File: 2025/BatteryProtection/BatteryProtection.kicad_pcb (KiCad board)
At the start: 2 copper layers, 58.4 x 140.1 mm, 57 parts, among them J1 Conn_01x02_Socket, J2 Conn_01x02_Pin, J3 Conn_01x02_Pin, Q1 IXTA140P05T, Q10 BC847, Q11 BC847, Q12 BC847, Q2 BC847, Q3 BC847, Q4 BC847, Q5 BC847, Q6 BC847, Q7 BC847, Q8 BC847, Q9 BC847, U1 MCP6561-OT, U2 MCP6561-OT, U3 MCP1799x-330xxTT

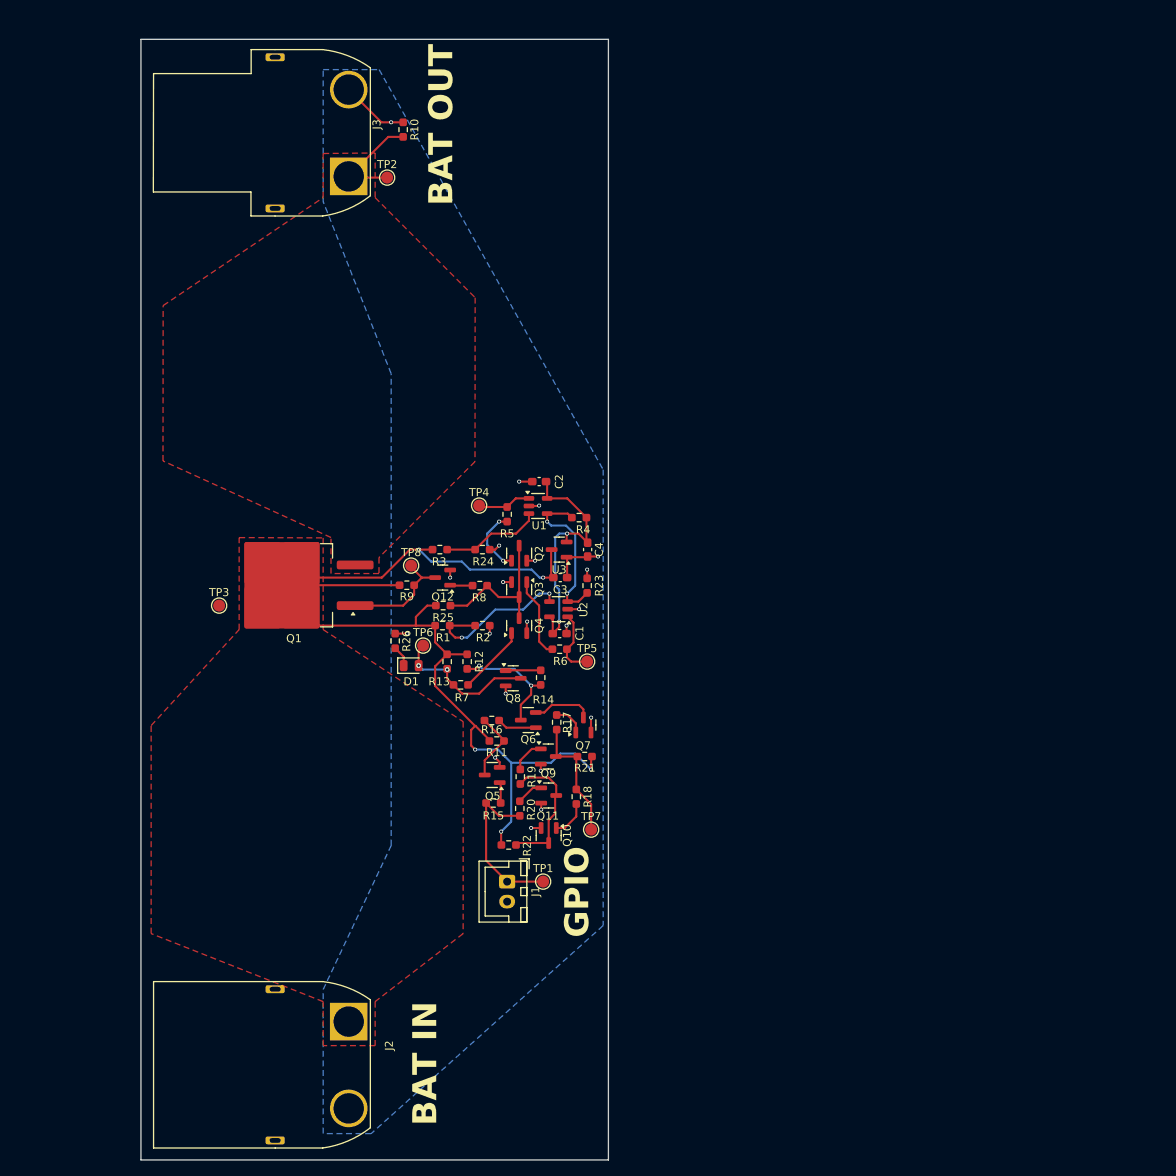
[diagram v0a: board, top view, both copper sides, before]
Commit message: DID the voltage protection PCB
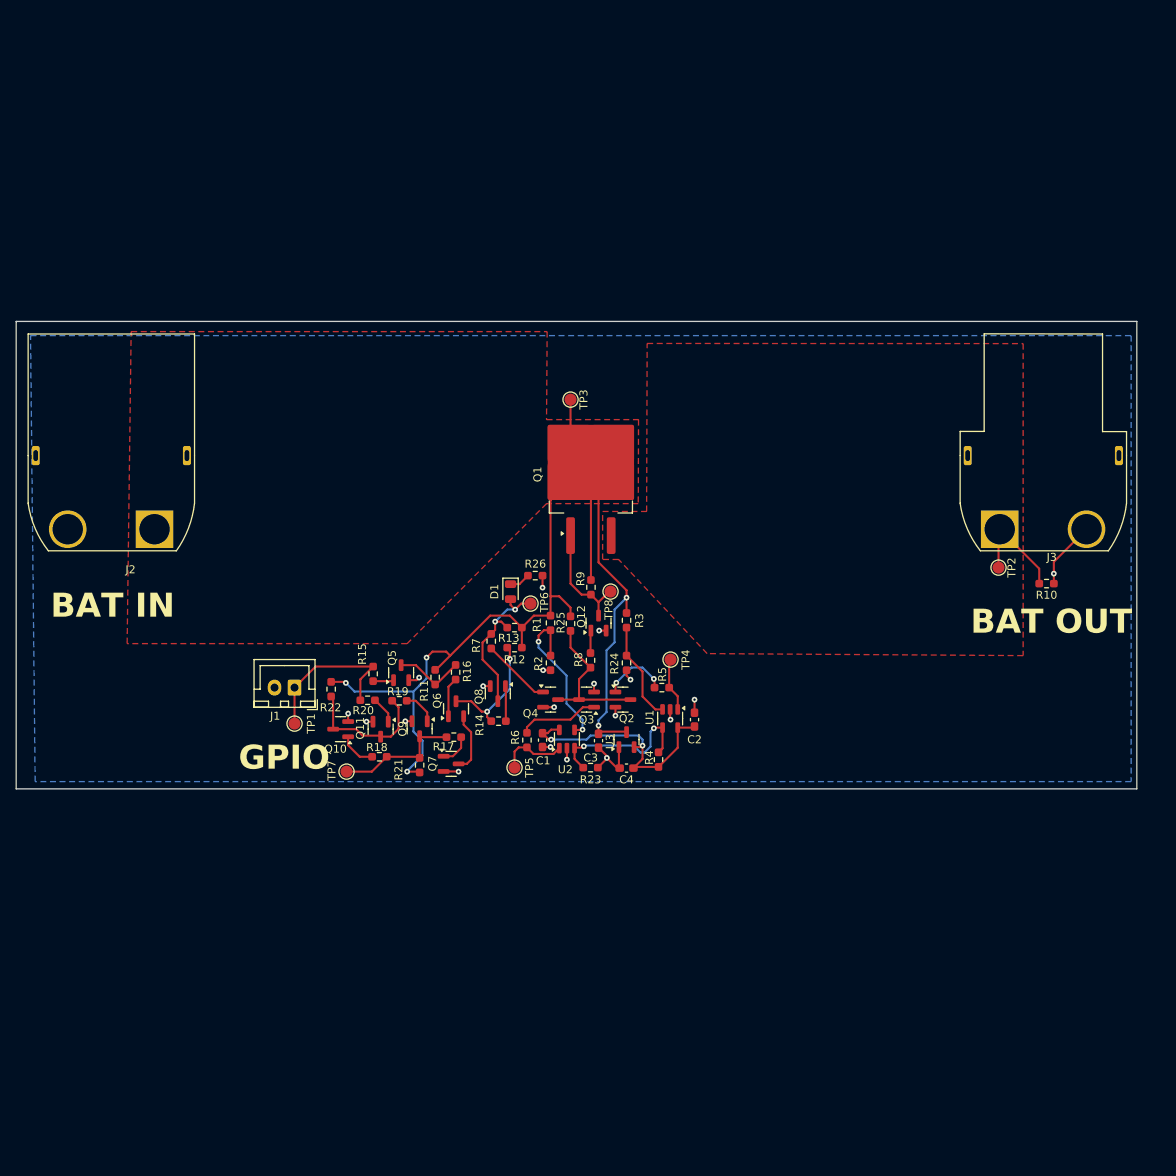
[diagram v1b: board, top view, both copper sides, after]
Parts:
- moved J3 104.7 mm to (257.9, 75.8), turned to 180 degrees
- moved R10 98.4 mm to (257.9, 91.8), turned to 180 degrees
- moved TP2 90.6 mm to (251.9, 89.8), turned to -90 degrees
- moved J2 78.4 mm to (141.4, 75.8), turned to 180 degrees
- moved TP3 50.9 mm to (198.4, 68.8), turned to -90 degrees
- moved Q1 39.6 mm to (201.0, 78.1), turned to 90 degrees
- moved TP1 36.8 mm to (163.9, 109.3), turned to -90 degrees
- moved J1 36.0 mm to (163.9, 104.8), turned to 180 degrees
- moved C2 35.5 mm to (213.9, 108.8), turned to -90 degrees
- moved R4 31.8 mm to (209.4, 113.8), turned to 90 degrees
- moved TP7 31.4 mm to (170.4, 115.3), turned to -90 degrees
- moved U1 31.3 mm to (210.9, 108.6), turned to -90 degrees
- moved TP4 30.7 mm to (210.9, 101.3), turned to -90 degrees
- moved R22 29.5 mm to (168.5, 104.9), turned to -90 degrees
- moved Q10 29.2 mm to (169.7, 109.9), turned to 180 degrees
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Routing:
- net Vs: track 130.4 -> 136.9 mm
- net Net-(D1-A): track 18.5 -> 20.1 mm
- net GND: track 37.1 -> 37.6 mm, vias 20 -> 19
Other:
- board size 58.4 x 140.1 mm -> 140.1 x 58.4 mm
